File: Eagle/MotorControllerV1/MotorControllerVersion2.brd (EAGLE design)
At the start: 50 x 60 mm, 33 parts, among them IC1 MC33932, IC2 74LVC1G04DCK, IC3 74LVC1G04DCK, IC4 7806DT

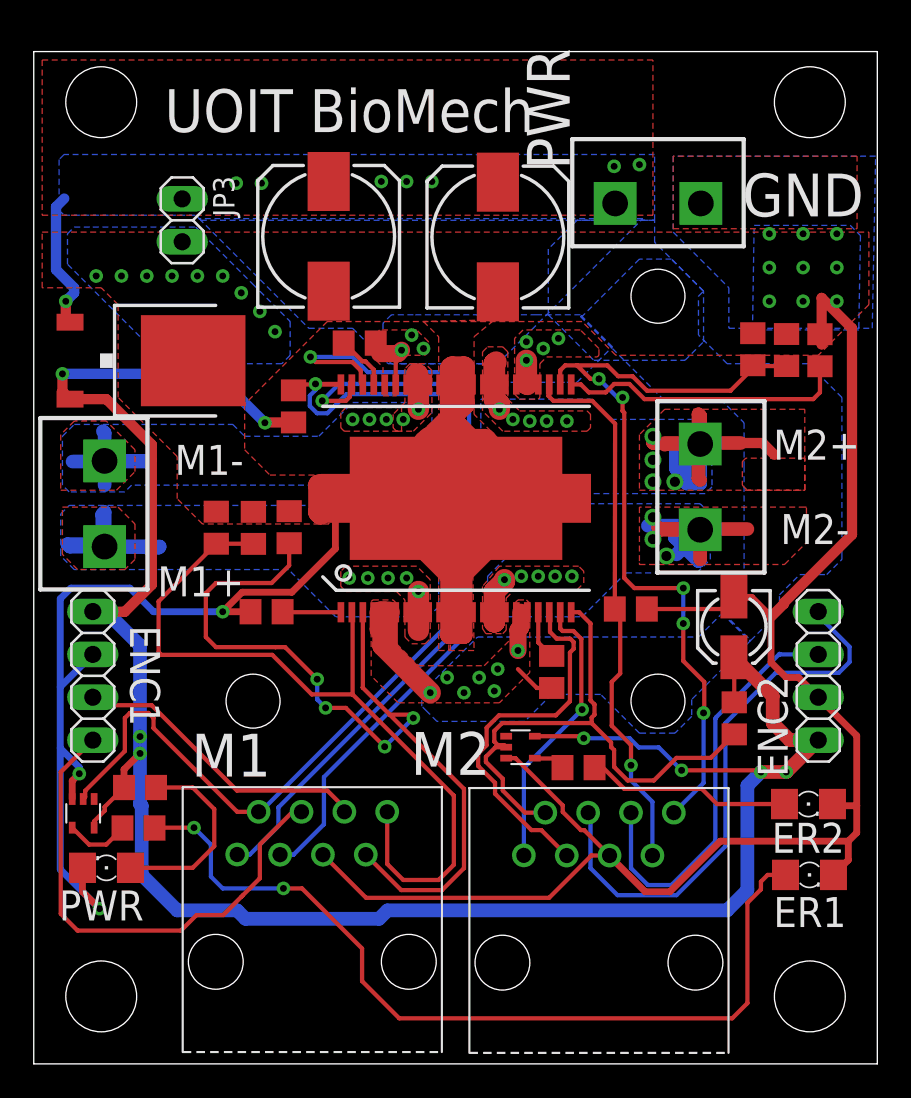
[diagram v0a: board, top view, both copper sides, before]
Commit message: Add files via upload
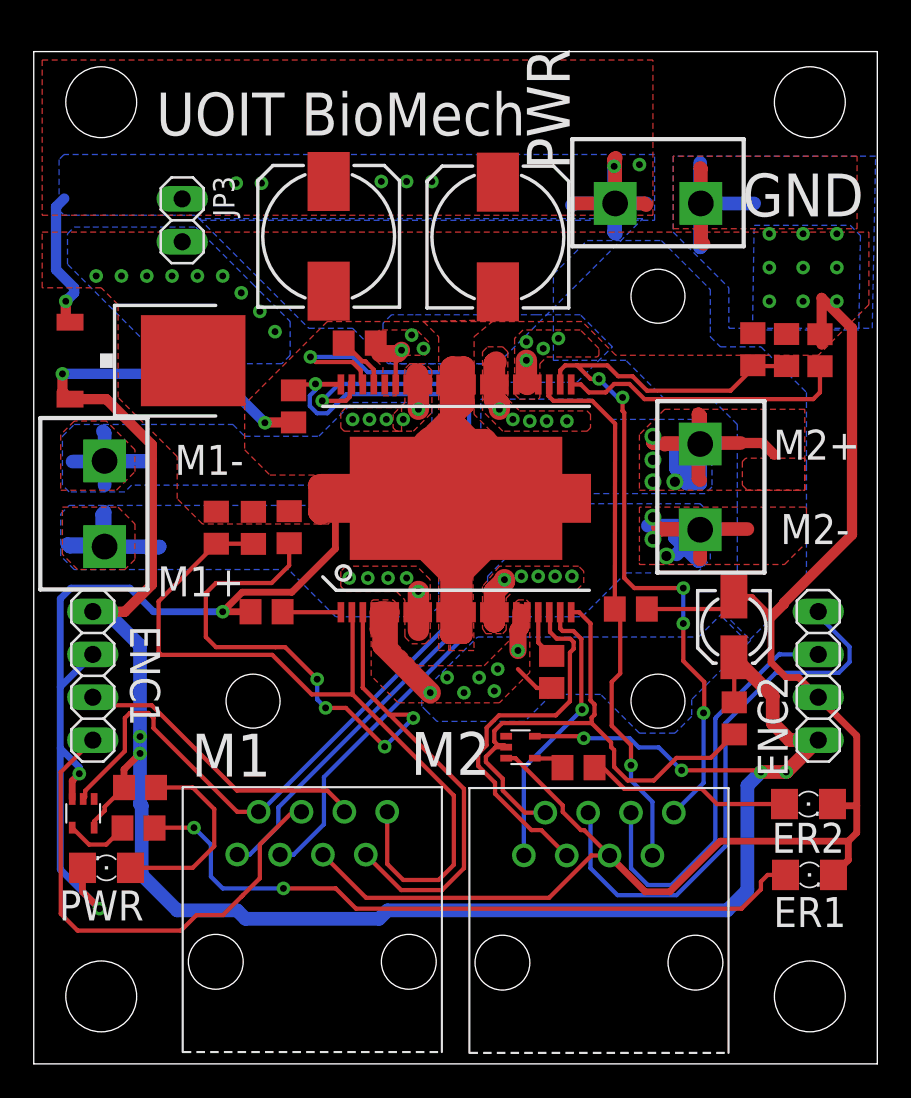
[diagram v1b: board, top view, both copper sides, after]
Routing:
- net VPWR: track 32.5 -> 50.2 mm
- net GND: track 204.3 -> 219.7 mm
- net N$15: track 51.6 -> 41.6 mm
- removed copper zone on layer 16, net PWR
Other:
- board text added: "1: IN1, 2: !SFA, 3: IN2, 4:ENCB 5:GND, 6:ENCA, 7: EN/!D2, 8: FBA"
- board text added: "BRAYDEN DEBOON 2019"
- board text added: "IC: MC33932"
- board text added: "MAX 5A"
- board text added: "V_IN 8-28V"
- board text removed: "LEGEND: 1 - IN1 2 - !SFA 3 - IN2 4 - ENCB* 5 - GND 6 - ENCA* 7 - EN/!D2 8 - FBA *If Encoder Connected IC: MC33932 **** 8 - 28 V **** Max 5A Brayden DeBoon 2018"
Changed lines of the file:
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@@
 <text x="11.7" y="18.3" size="2.54" layer="21" ratio="10" align="center">M1 </text>
 <text x="24.7" y="18.4" size="2.54" layer="21" ratio="10" align="center">M2</text>
-<text x="18.7" y="56.5" size="2.54" layer="21" ratio="10" align="center">UOIT BioMech</text>
-<text x="25" y="33.5" size="2.54" layer="22" ratio="10" rot="MR0" align="center">LEGEND:
-1 - IN1       2 - !SFA
-3 - IN2       4 - ENCB*
-5 - GND      6 - ENCA*
-7 - EN/!D2  8 - FBA
-*If Encoder Connected
-IC: MC33932
-**** 8 - 28 V ****
-Max 5A
-Brayden DeBoon 2018</text>
+<text x="18.2" y="56.3" size="2.54" layer="21" ratio="10" align="center">UOIT BioMech</text>
+<text x="40.3" y="54.8" size="1.4224" layer="22" rot="MR0">1: IN1, 2: !SFA, 3: IN2, 4:ENCB
+5:GND, 6:ENCA, 7: EN/!D2, 8: FBA</text>
+<text x="31.3" y="34.7" size="1.4224" layer="22" rot="MR0">IC: MC33932</text>
+<text x="29.4" y="48.3" size="1.4224" layer="22" rot="MR0">V_IN 8-28V</text>
+<text x="29.4" y="45.6" size="1.4224" layer="22" rot="MR0">MAX 5A</text>
+<text x="34.9" y="31.3" size="1.4224" layer="22" rot="MR0">BRAYDEN DEBOON 2019</text>
 </plain>
 <attributes>
@@
 </polygon>
 <via x="43.6" y="45.2" extent="1-16" drill="0.4064"/>
+<wire x1="39.54" y1="51" x2="39.54" y2="48.44" width="0.8128" layer="16"/>
+<wire x1="39.54" y1="48.44" x2="39.5" y2="48.4" width="0.8128" layer="16"/>
+<wire x1="39.5" y1="48.4" x2="39.5" y2="51.04" width="0.8128" layer="16"/>
+<wire x1="39.5" y1="53.4" x2="39.5" y2="51.04" width="0.8128" layer="16"/>
+<wire x1="39.5" y1="51.04" x2="39.54" y2="51" width="0.8128" layer="16"/>
+<wire x1="42.7" y1="51" x2="39.54" y2="51" width="0.8128" layer="16"/>
+<wire x1="39.7" y1="48.6" x2="39.54" y2="48.76" width="0.8128" layer="1"/>
+<wire x1="39.54" y1="48.76" x2="39.54" y2="51" width="0.8128" layer="1"/>
+<wire x1="39.5" y1="53.1" x2="39.54" y2="53.06" width="0.8128" layer="1"/>
+<wire x1="39.54" y1="53.06" x2="39.54" y2="51" width="0.8128" layer="1"/>
 </signal>
 <signal name="IN1">
@@
 <wire x1="9.5" y1="14" x2="7.18" y2="14" width="0.254" layer="1"/>
 <via x="14.8" y="10.4" extent="1-16" drill="0.4064"/>
-<wire x1="14.8" y1="10.4" x2="15.9" y2="10.4" width="0.254" layer="1"/>
-<wire x1="19.462" y1="6.838" x2="19.462" y2="4.90345625" width="0.254" layer="1"/>
-<wire x1="19.462" y1="4.90345625" x2="21.66545625" y2="2.7" width="0.254" layer="1"/>
-<wire x1="21.66545625" y1="2.7" x2="41.4" y2="2.7" width="0.254" layer="1"/>
-<wire x1="15.9" y1="10.4" x2="19.462" y2="6.838" width="0.254" layer="1"/>
-<wire x1="41.4" y1="2.7" x2="42.3" y2="3.6" width="0.254" layer="1"/>
-<wire x1="42.3" y1="3.6" x2="42.3" y2="9.542" width="0.254" layer="1"/>
-<wire x1="42.3" y1="9.542" x2="43.1" y2="10.342" width="0.254" layer="1"/>
 <wire x1="43.1" y1="10.342" x2="43.1" y2="10.8" width="0.254" layer="1"/>
 <wire x1="43.1" y1="10.8" x2="43.5" y2="11.2" width="0.254" layer="1"/>
 <wire x1="43.5" y1="11.2" x2="44.558" y2="11.2" width="0.254" layer="1"/>
+<wire x1="17.9" y1="10.4" x2="19.1" y2="9.2" width="0.254" layer="1"/>
+<wire x1="19.1" y1="9.2" x2="41.958" y2="9.2" width="0.254" layer="1"/>
+<wire x1="14.8" y1="10.4" x2="17.9" y2="10.4" width="0.254" layer="1"/>
+<wire x1="41.958" y1="9.2" x2="43.1" y2="10.342" width="0.254" layer="1"/>
 </signal>
 <signal name="N$16">
@@
 <wire x1="21.455" y1="40.27" x2="21.455" y2="41.955" width="0.254" layer="1"/>
 <wire x1="21.455" y1="41.955" x2="21.8" y2="42.3" width="0.254" layer="1"/>
-<wire x1="21.455" y1="40.27" x2="21.0668" y2="26.77" width="0" layer="19" extent="1-1"/>
+<wire x1="34.46" y1="51" x2="34.46" y2="53.66" width="0.8128" layer="1"/>
+<wire x1="34.46" y1="53.66" x2="34.5" y2="53.7" width="0.8128" layer="1"/>
+<wire x1="34.46" y1="53.66" x2="34.4" y2="53.6" width="0.8128" layer="1"/>
+<wire x1="34.4" y1="53.6" x2="34.4" y2="53.2" width="0.8128" layer="1"/>
+<wire x1="32" y1="51" x2="34.46" y2="51" width="0.8128" layer="1"/>
+<wire x1="36.3" y1="50.9" x2="36.2" y2="51" width="0.8128" layer="1"/>
+<wire x1="36.2" y1="51" x2="34.46" y2="51" width="0.8128" layer="1"/>
+<wire x1="34.46" y1="51" x2="34.46" y2="49.24" width="0.8128" layer="16"/>
+<wire x1="34.46" y1="49.24" x2="34.5" y2="49.2" width="0.8128" layer="16"/>
+<wire x1="34.46" y1="49.24" x2="34.4" y2="49.3" width="0.8128" layer="16"/>
+<wire x1="34.4" y1="49.3" x2="34.4" y2="51" width="0.8128" layer="16"/>
+<wire x1="34.4" y1="51" x2="34.4" y2="53.2" width="0.8128" layer="16"/>
+<wire x1="32" y1="51" x2="31.9" y2="50.9" width="0.8128" layer="16"/>
+<wire x1="32" y1="51" x2="34.4" y2="51" width="0.8128" layer="16"/>
+<wire x1="36.3" y1="51" x2="34.4" y2="51" width="0.8128" layer="16"/>
+<polygon width="0.35" layer="16">
+<vertex x="40.8" y="26.6"/>
+<vertex x="41.7" y="27.5"/>
+<vertex x="41.7" y="33"/>
+<vertex x="41.7" y="37.9"/>
+<vertex x="40.9" y="38.7"/>
+<vertex x="40.2" y="39.4"/>
+<vertex x="37.4" y="39.4"/>
+<vertex x="35.1" y="41.7"/>
+<vertex x="30.8" y="41.7"/>
+<vertex x="30.8" y="46.8"/>
+<vertex x="32.8" y="48.8"/>
+<vertex x="37.2" y="48.8"/>
+<vertex x="40" y="46"/>
+<vertex x="40.1" y="45.9"/>
+<vertex x="40.1" y="43.7"/>
+<vertex x="40.1" y="43.1"/>
+<vertex x="40.7" y="42.5"/>
+<vertex x="43.1" y="42.5"/>
+<vertex x="45.8" y="39.8"/>
+<vertex x="45.8" y="35.5"/>
+<vertex x="45.8" y="28.7"/>
+<vertex x="44.3" y="27.2"/>
+<vertex x="44.3" y="27"/>
+<vertex x="42.3" y="25"/>
+<vertex x="40.8" y="26.5"/>
+</polygon>
 </signal>
 <signal name="ENC1_A">
@@
 <wire x1="33" y1="14.75" x2="32.86" y2="14.89" width="0.254" layer="16"/>
 </signal>
-<signal name="PWR">
-<polygon width="0.254" layer="16">
-<vertex x="34.3" y="42.4"/>
-<vertex x="37.3" y="39.4"/>
-<vertex x="40.7" y="39.4"/>
-<vertex x="42.1" y="38"/>
-<vertex x="42.1" y="35.4"/>
-<vertex x="42.1" y="28"/>
-<vertex x="40.8" y="26.7"/>
-<vertex x="42.4" y="25.1"/>
-<vertex x="42.5" y="25.1"/>
-<vertex x="44.2" y="26.8"/>
-<vertex x="44.2" y="27.8"/>
-<vertex x="45.4" y="29"/>
-<vertex x="47" y="29"/>
-<vertex x="47.9" y="29.9"/>
-<vertex x="47.9" y="30.1"/>
-<vertex x="47.9" y="39.5"/>
-<vertex x="45.9" y="41.5"/>
-<vertex x="41.1" y="41.5"/>
-<vertex x="39.4" y="43.2"/>
-<vertex x="39.4" y="45.5"/>
-<vertex x="39.7" y="45.8"/>
-<vertex x="37.8" y="47.7"/>
-<vertex x="35.9" y="47.7"/>
-<vertex x="32.5" y="44.3"/>
-<vertex x="32.4" y="44.3"/>
-</polygon>
-<polygon width="0.254" layer="16">
-<vertex x="30.5" y="44.4"/>
-<vertex x="33.2" y="41.7"/>
-<vertex x="38.6" y="41.7"/>
-<vertex x="39.7" y="42.8"/>
-<vertex x="39.7" y="45.8"/>
-<vertex x="36.8" y="48.7"/>
-<vertex x="36.8" y="50"/>
-<vertex x="32.2" y="50"/>
-<vertex x="32.1" y="49.9"/>
-<vertex x="30.5" y="48.3"/>
-</polygon>
-</signal>
 </signals>
-<errors>
-</errors>
 </board>
 </drawing>
